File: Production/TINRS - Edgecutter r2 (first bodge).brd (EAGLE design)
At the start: 59.6 x 106.5 mm, 168 parts, among them IC1 LD1117AS33TR, IC10 MCP4822-E/SN, IC2 MCP6004, IC3 TL074D, IC4 MCP6004, IC5 MKL02Z32VFK4, IC6 24LC16T-I/OT, IC7 74HC595BQ, IC8 74HC595BQ, IC9 74HC595BQ, J1 PJ-341, J10 PJ-341, J11 PJ-341, J12 PJ-341, J13 PJ-341, J14 POWERSMT, J15 PJ-341, J2 PJ-341, J3 PJ-341, J4 PJ-341, J5 PJ-341, J6 PJ-341, J7 PJ-341, J8 PJ-341, J9 PJ-341, Q1 MMBT3904, Q2 MMBT3904, Q3 MMBT3904, Q4 MMBT3904, Q7 MMBT3904, Q8 MMBT3904, U2 LM4040DIM3-5.0

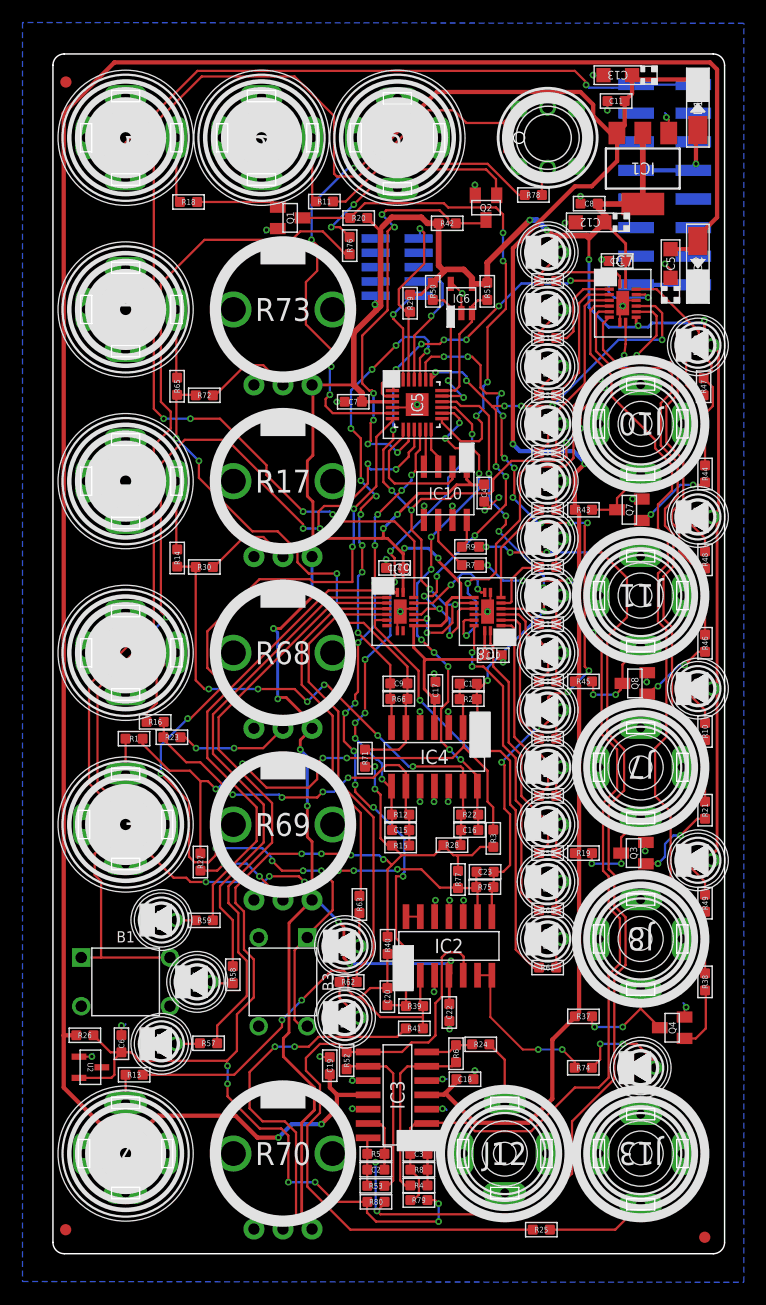
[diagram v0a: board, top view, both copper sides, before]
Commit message: Tuesday + library updates
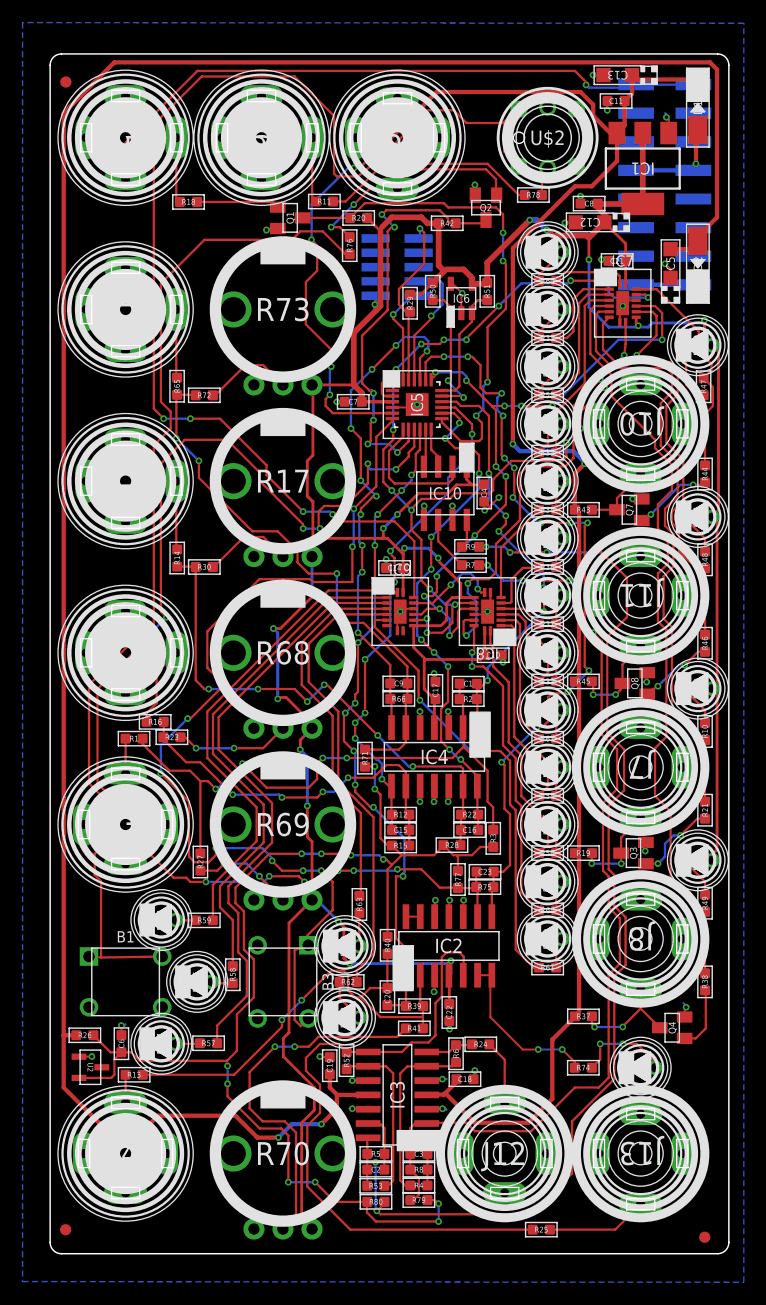
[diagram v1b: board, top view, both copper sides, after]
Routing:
- net BUTTON_TIMERANGE: track 91.4 -> 90.0 mm
- net BUTTON_LOOP: track 84.9 -> 85.7 mm
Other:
- board size 59.6 x 106.5 mm -> 60.2 x 106.5 mm
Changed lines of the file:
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@@
 <contactref element="B1" pad="4"/>
 <contactref element="IC5" pad="9"/>
-<wire x1="3.683" y1="26.289" x2="5.44355" y2="26.289" width="0.2032" layer="1"/>
-<wire x1="5.44355" y1="26.289" x2="11.557" y2="26.289" width="0.2032" layer="1"/>
+<wire x1="4.37" y1="26.38" x2="5.44355" y2="26.289" width="0.2032" layer="1"/>
+<wire x1="5.44355" y1="26.289" x2="10.87" y2="26.38" width="0.2032" layer="1"/>
 <wire x1="33.246" y1="73.175" x2="33.246" y2="71.621" width="0.2032" layer="1"/>
 <wire x1="33.246" y1="71.621" x2="32.75" y2="71.125" width="0.2032" layer="1"/>
@@
 <contactref element="B3" pad="4"/>
 <contactref element="IC5" pad="6"/>
-<wire x1="23.749" y1="20.193" x2="23.182" y2="20.193" width="0.2032" layer="1"/>
+<wire x1="23.84" y1="20.88" x2="23.182" y2="20.193" width="0.2032" layer="1"/>
 <wire x1="23.182" y1="20.193" x2="22.625" y2="20.75" width="0.2032" layer="1"/>
 <wire x1="22.625" y1="20.75" x2="22.625" y2="26.943" width="0.2032" layer="1"/>
-<wire x1="22.625" y1="26.943" x2="23.749" y2="28.067" width="0.2032" layer="1"/>
+<wire x1="22.625" y1="26.943" x2="23.84" y2="27.38" width="0.2032" layer="1"/>
 <wire x1="31.3" y1="74.1304" x2="31.3" y2="73.925" width="0.2032" layer="1"/>
 <wire x1="31.3" y1="73.925" x2="29.875" y2="72.5" width="0.2032" layer="1"/>
@@
 <wire x1="24" y1="59.875" x2="19.5" y2="59.875" width="0.2032" layer="1"/>
 <wire x1="19.5" y1="59.875" x2="14.875" y2="55.25" width="0.2032" layer="1"/>
-<wire x1="23.749" y1="28.067" x2="23.749" y2="28.249" width="0.2032" layer="1"/>
+<wire x1="23.84" y1="27.38" x2="23.749" y2="28.249" width="0.2032" layer="1"/>
 <wire x1="23.749" y1="28.249" x2="26" y2="30.5" width="0.2032" layer="1"/>
 <wire x1="26" y1="30.5" x2="26" y2="33" width="0.2032" layer="1"/>
